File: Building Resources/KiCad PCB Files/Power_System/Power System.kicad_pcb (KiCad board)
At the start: 2 copper layers, 45.8 x 37.9 mm, 15 parts, among them J1 Conn_01x02_Socket, J2 Conn_01x02_Socket, J3 Conn_01x02_Socket, J4 Conn_01x02_Socket, J5 Conn_01x02_Socket, U1 LM2596T-3.3

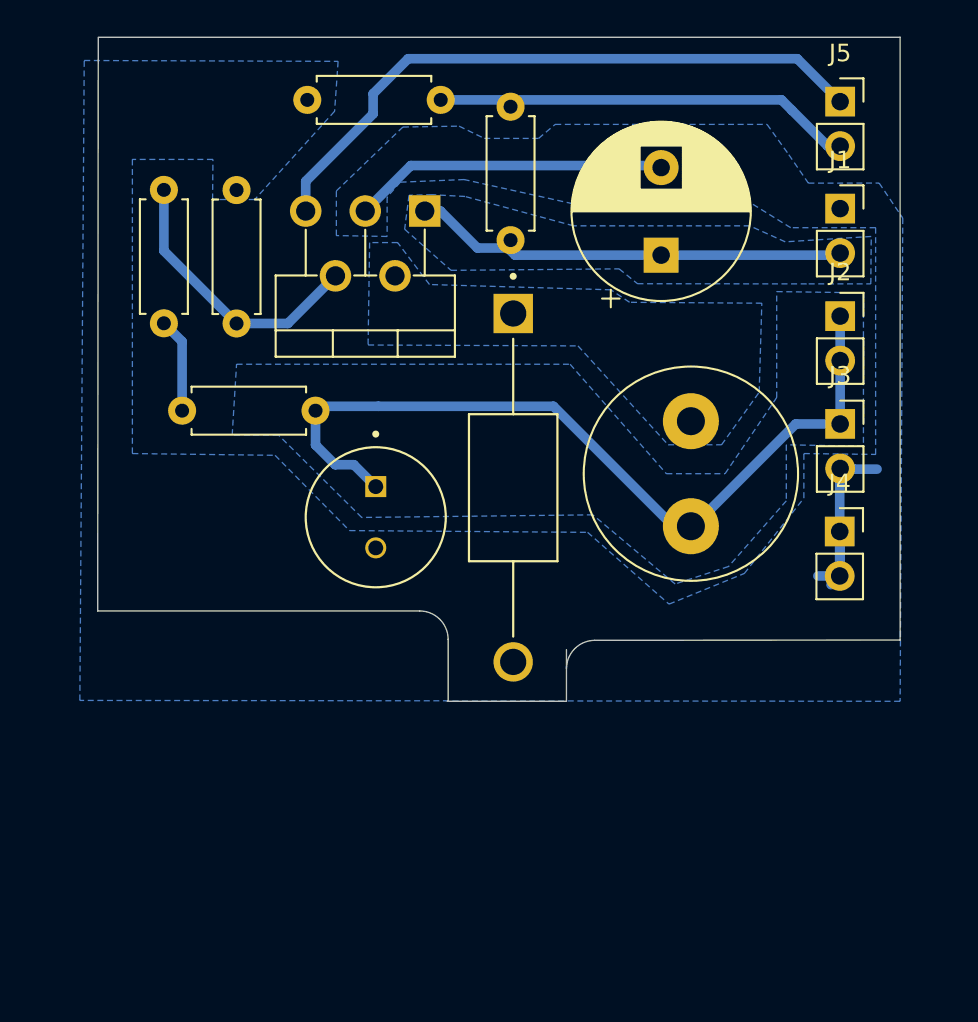
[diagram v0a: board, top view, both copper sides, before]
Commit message: Update KiCad Files (#59)
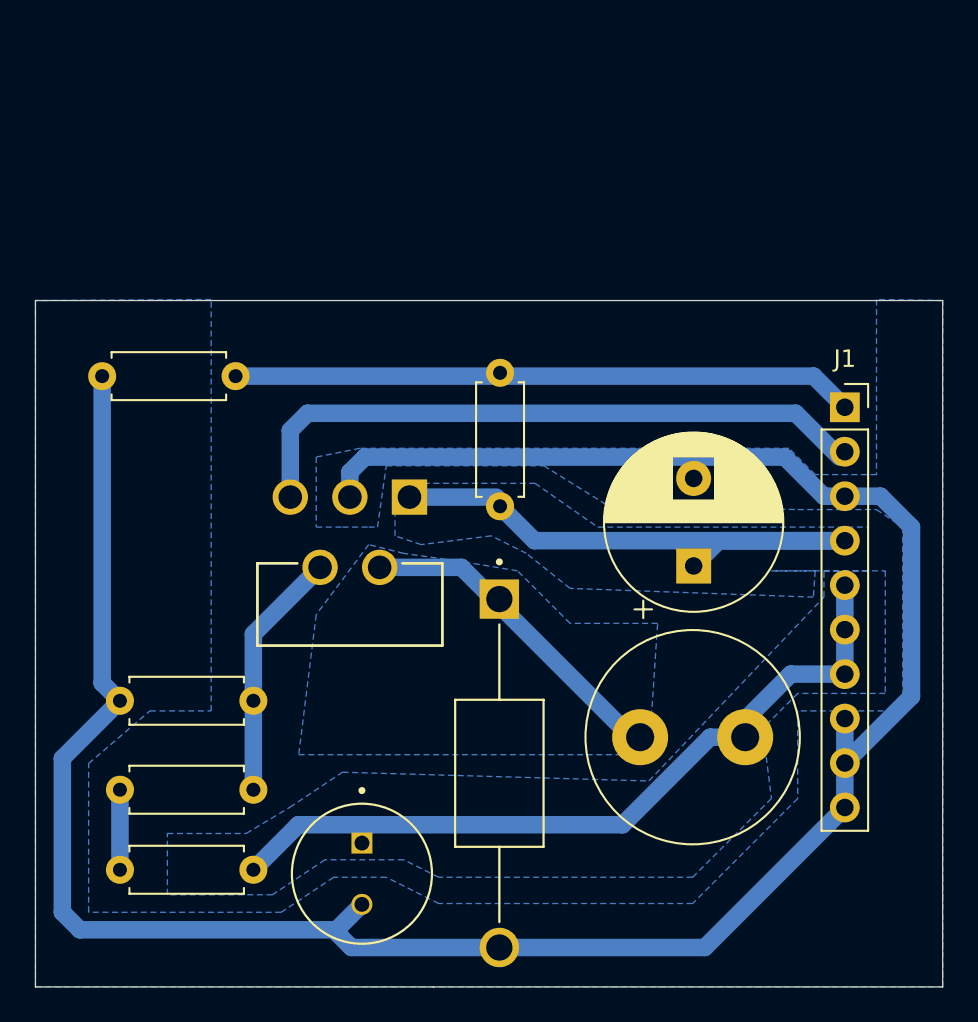
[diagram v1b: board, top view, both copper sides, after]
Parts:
- removed J2, J3, J4, J5: Conn_01x02_Socket, Connector_PinSocket_2.54mm:PinSocket_1x02_P2.54mm_Vertical
- C2: value 220u -> 220uF
- J1: value Conn_01x02_Socket -> Conn_01x10; footprint Connector_PinSocket_2.54mm:PinSocket_1x02_P2.54mm_Vertical -> Connector_PinSocket_2.54mm:PinSocket_1x10_P2.54mm_Vertical
- L1: value 68m -> 68mH
- R2-1: value 18k -> 1.6k
- R2-2: value 120k -> 1.6k
- R3: value 82k -> 1k
- U1: footprint Package_TO_SOT_THT:TO-220-5_P3.4x3.7mm_StaggerOdd_Lead3.8mm_Vertical -> LM2596TVADJG:TO170P470X1016X2092-5P
- moved R2-1 34.6 mm to (168.9, 63.5), turned to 180 degrees
- moved R3 29.9 mm to (161.3, 58.4), turned to 0 degrees
- moved R2-2 26.5 mm to (161.3, 68.1)
- moved C2 20.4 mm to (175.1, 68.3)
- moved R2 19.7 mm to (167.9, 39.9)
- moved C1 17.8 mm to (194.1, 50.7)
- moved D1 16.3 mm to (183.0, 62.6)
- moved R1 15.2 mm to (183.0, 47.3)
- moved L1 12.4 mm to (197.0, 60.5), turned to 180 degrees
- moved U1 12.1 mm to (177.4, 42.5), turned to 0 degrees
- moved J1 11.3 mm to (202.7, 41.7)
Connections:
- C2 pad 1: Net-(J2-Pin_1) -> Net-(J1-Pin_5)
- J1 pad 1: GNDREF -> Net-(J1-Pin_1)
- J1 pad 2: +6V -> Net-(J1-Pin_2)
- L1 pad 1: Net-(J2-Pin_1) -> Net-(J1-Pin_5)
- R1 pad 2: Net-(J5-Pin_2) -> Net-(J1-Pin_1)
- R2 pad 1: Net-(J5-Pin_2) -> Net-(J1-Pin_1)
- R2-2 pad 2: Net-(J2-Pin_1) -> Net-(J1-Pin_5)
- U1 pad 5: Net-(J5-Pin_1) -> Net-(J1-Pin_2)
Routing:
- net GNDREF: track 31.0 -> 139.1 mm
- net Net-(J2-Pin_1): track 47.9 -> 0.00 mm
- net Net-(J1-Pin_5): track 0.00 -> 43.5 mm
- net Net-(J5-Pin_1): track 36.8 -> 0.00 mm
- net Net-(J1-Pin_2): track 0.00 -> 36.6 mm
- net Net-(J1-Pin_1): track 0.00 -> 35.5 mm
- net Net-(J5-Pin_2): track 23.9 -> 0.00 mm
- net Net-(D1-K): track 0.95 -> 18.2 mm
- net +6V: track 24.8 -> 34.7 mm
- net Net-(U1-FB): track 16.1 -> 14.3 mm
- net Net-(R2-1-Pad2): track 5.42 -> 4.57 mm
- added copper zone on B.Cu, net Net-(J1-Pin_5)
- removed copper zone on B.Cu, net Net-(J2-Pin_1)
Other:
- board size 45.8 x 37.9 mm -> 51.8 x 39.2 mm
